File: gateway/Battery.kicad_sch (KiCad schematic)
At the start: 31 parts, among them IC901 BQ25300, IC902 MAX17048, IC903 BQ297xy, Q901 CSD16301Q2, Q902 CSD16301Q2

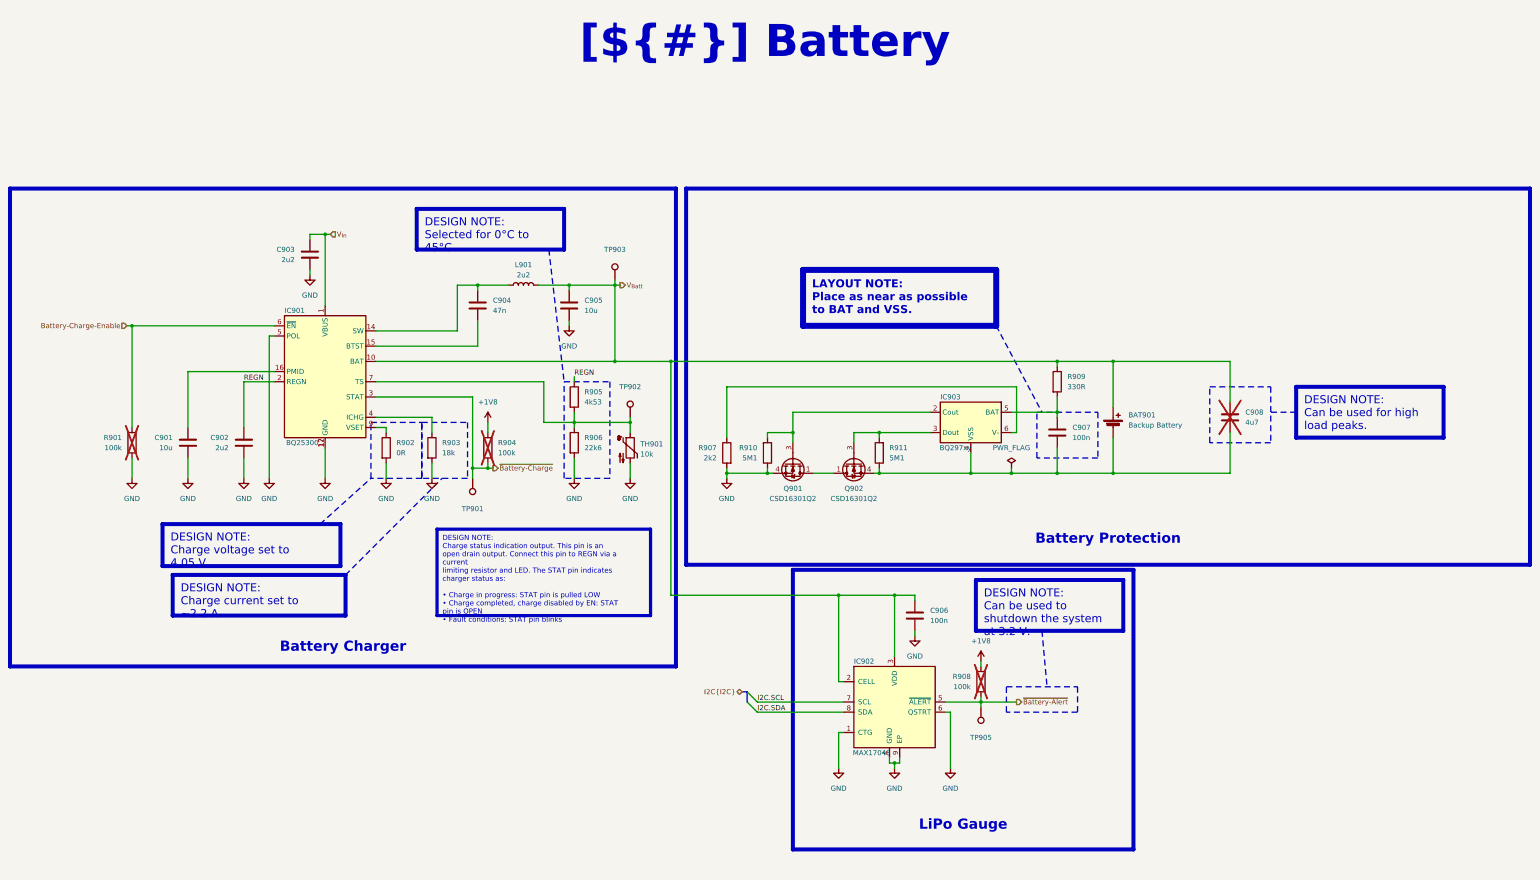
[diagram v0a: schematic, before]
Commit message: Working on revision 1.0.0
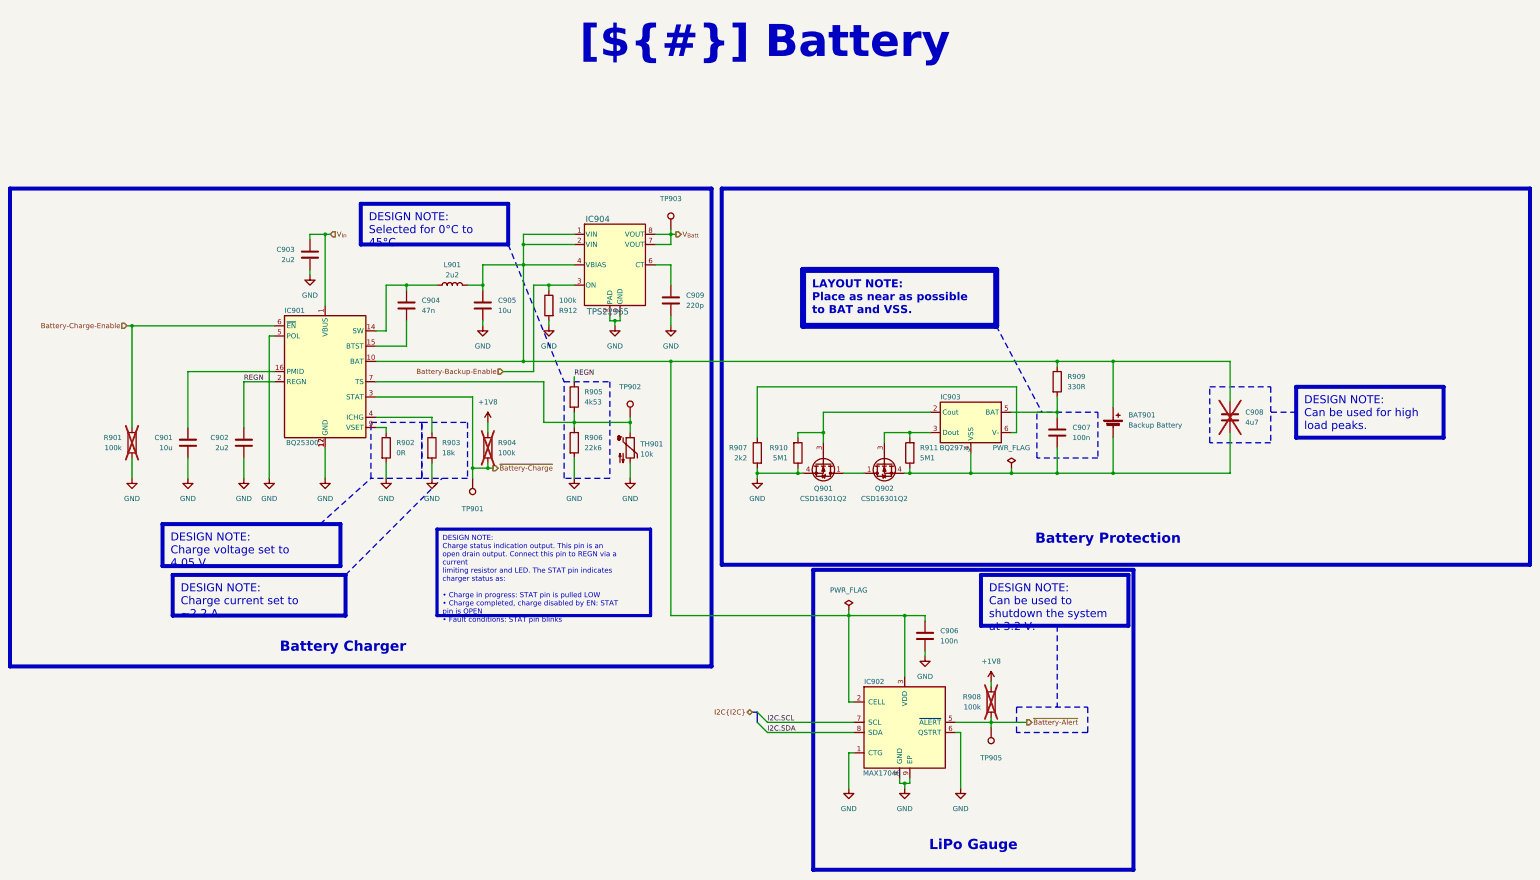
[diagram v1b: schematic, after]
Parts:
- added C909: 220p, Capacitor_SMD:C_0805_2012Metric, symbol Device:C
- added IC904: TPS22965, Package_SON:WSON-8-1EP_2x2mm_P0.5mm_EP0.9x1.6mm_ThermalVias, symbol Texas Instruments:TPS22965
- added R912: 100k, Resistor_SMD:R_0805_2012Metric, symbol partdb:RT0805FRE13100KL
- C901, C905: symbol Device:C -> partdb:0805X7R106KT1AT; Category (none) -> Kondensator/MLCC; MPN (none) -> 0805X7R106KT1AT; Manufacturer (none) -> KYOCERA AVX; Manufacturing Status (none) -> Active; Mouser SPN (none) -> 581-0805X7R106KT1AT; Part-DB Footprint (none) -> 0805; Part-DB ID (none) -> 331; Part-DB URL (none) -> https://inventory.lan/de/part/331/info; Stock (none) -> 0
- C902, C903: symbol Device:C -> partdb:MCJCT21GCB7225MTPA1J; Category (none) -> Kondensator/MLCC; MPN (none) -> MCJCT21GCB7225MTPA1J; Manufacturer (none) -> TAIYO YUDEN; Manufacturing Status (none) -> Active; Mouser SPN (none) -> 963-T21GCB7225MTPA1J; Part-DB Footprint (none) -> 0805; Part-DB ID (none) -> 328; Part-DB URL (none) -> https://inventory.lan/de/part/328/info; Stock (none) -> 0; manf KYOCERA AVX -> TAIYO YUDEN; manf# 0805ZC225JAT2A -> MCJCT21GCB7225MTPA1J; mouser# 581-0805ZC225JAT2A -> 963-T21GCB7225MTPA1J
- C906, C907: symbol Device:C -> partdb:08055C104K4Z4A; Category (none) -> Kondensator/MLCC; MPN (none) -> 08055C104K4Z4A; Manufacturer (none) -> KYOCERA AVX; Manufacturing Status (none) -> Active; Mass (none) -> 0.006 g; Mouser SPN (none) -> 581-08055C104K4Z4A; Part-DB Footprint (none) -> 0805; Part-DB ID (none) -> 109; Part-DB URL (none) -> https://inventory.lan/de/part/109/info; Stock (none) -> 6; Storage Location (none) -> Sortierregal; manf# 08053C104M4T4A -> 08055C104K4Z4A; mouser# 581-08053C104M4T4A -> 581-08055C104K4Z4A
- IC902: Category (none) -> IC/Sensor; MPN (none) -> MAX17048G+T10; Manufacturer (none) -> Analog Devices / Maxim Integrated; Mass (none) -> 0.05 g; Mouser SPN (none) -> 700-MAX17048G+T10; Part-DB Footprint (none) -> TDFN-8-1EP_2x2mm_P0.5mm_EP0.8x1.2mm; Part-DB ID (none) -> 273; Part-DB URL (none) -> https://inventory.lan/de/part/273/info; Stock (none) -> 0
- R901, R904, R908: symbol Device:R -> partdb:RT0805FRE13100KL; Category (none) -> Widerstand/Dünnfilmwiderstand; MPN (none) -> RT0805FRE13100KL; Manufacturer (none) -> YAGEO; Manufacturing Status (none) -> Active; Mass (none) -> 0.006 g; Mouser SPN (none) -> 603-RT0805FRE13100KL; Part-DB Footprint (none) -> 0805; Part-DB ID (none) -> 66; Part-DB URL (none) -> https://inventory.lan/de/part/66/info; Stock (none) -> 4; Storage Location (none) -> Sortierregal; manf Bourns -> YAGEO; manf# CR0805-JW-104GLF -> RT0805FRE13100KL; mouser# 652-CR0805-JW-104GLF -> 603-RT0805FRE13100KL
- R902: symbol Device:R -> partdb:CR0805-J/-000ELF; Category (none) -> Widerstand/Dickfilmwiderstand; MPN (none) -> CR0805-J/-000ELF; Manufacturer (none) -> Bourns; Manufacturing Status (none) -> Active; Mass (none) -> 0.006 g; Mouser SPN (none) -> 652-CR0805-J/-000ELF; Part-DB Footprint (none) -> 0805; Part-DB ID (none) -> 322; Part-DB URL (none) -> https://inventory.lan/de/part/322/info; Stock (none) -> 0
- R907: symbol Device:R -> partdb:CR0805-JW-222ELF; Category (none) -> Widerstand/Dickfilmwiderstand; MPN (none) -> CR0805-JW-222ELF; Manufacturer (none) -> Bourns; Manufacturing Status (none) -> Active; Mass (none) -> 0.006 g; Mouser SPN (none) -> 652-CR0805JW-222ELF; Part-DB Footprint (none) -> 0805; Part-DB ID (none) -> 72; Part-DB URL (none) -> https://inventory.lan/de/part/72/info; Stock (none) -> 50; Storage Location (none) -> Sortierregal; mouser# 652-CR0805-JW-222ELF -> 652-CR0805JW-222ELF
- R909: symbol Device:R -> partdb:CR0805-JW-331ELF; Category (none) -> Widerstand/Dickfilmwiderstand; MPN (none) -> CR0805-JW-331ELF; Manufacturer (none) -> Bourns; Manufacturing Status (none) -> Active; Mass (none) -> 0.006 g; Mouser SPN (none) -> 652-CR0805JW-331ELF; Part-DB Footprint (none) -> 0805; Part-DB ID (none) -> 323; Part-DB URL (none) -> https://inventory.lan/de/part/323/info; Stock (none) -> 0; manf# CR0805-JW-331GLF -> CR0805-JW-331ELF; mouser# 652-CR0805-JW-331GLF -> 652-CR0805JW-331ELF
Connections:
- net GND: now also C909.2, IC904.5 (GND), IC904.9 (PAD), R912.2
- net V_{Batt}: now also IC904.7 (VOUT), IC904.8 (VOUT); no longer BAT901.1 (+), C905.1, C906.1, C908.1, IC901.10 (BAT), IC902.2 (CELL), IC902.3 (VDD), L901.2, R909.1
- new net: BAT901.1 (+), C905.1, C906.1, C908.1, IC901.10 (BAT), IC902.2 (CELL), IC902.3 (VDD), IC904.1 (VIN), IC904.2 (VIN), IC904.4 (VBIAS), L901.2, R909.1
- new net: C909.1, IC904.6 (CT)
- new net Battery-Backup-Enable: IC904.3 (ON), R912.1
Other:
- moved on the sheet: C904, C905, C906, IC902, L901, Q901, Q902, R907, R908, R910, R911, TP903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
